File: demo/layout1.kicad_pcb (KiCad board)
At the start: 2 copper layers, 38 x 14 mm, 28 parts, among them J1 MICRO-USB-B-alt, P1 CONN_01X06, U1 FTDI-FT230X, U2 MCP1703-alt

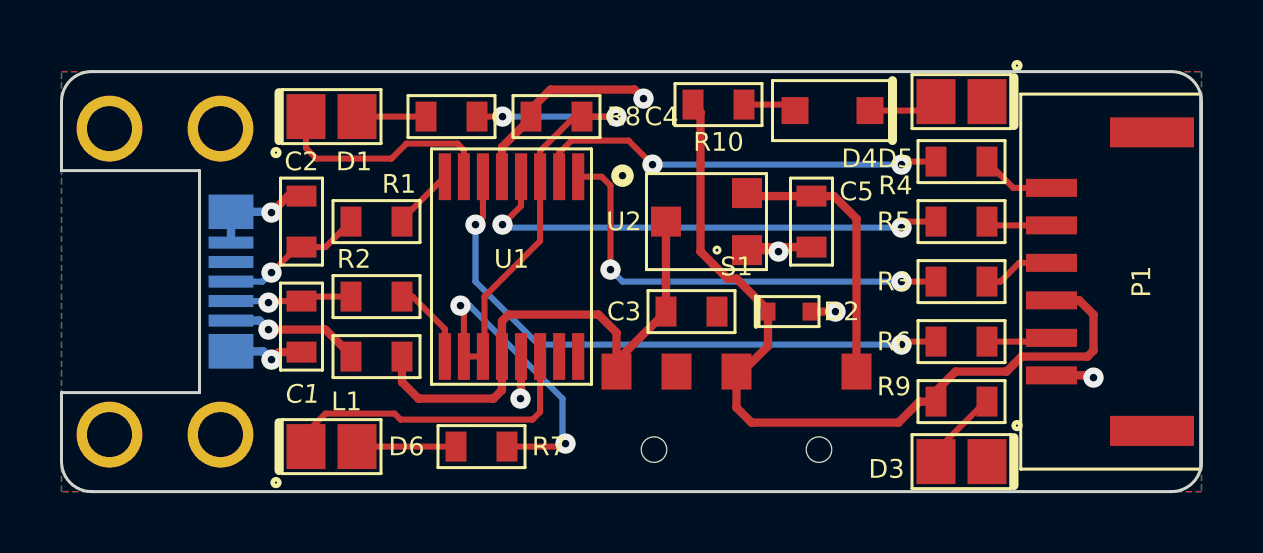
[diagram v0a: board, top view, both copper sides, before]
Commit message: lots of changes, can recenter placement,etc
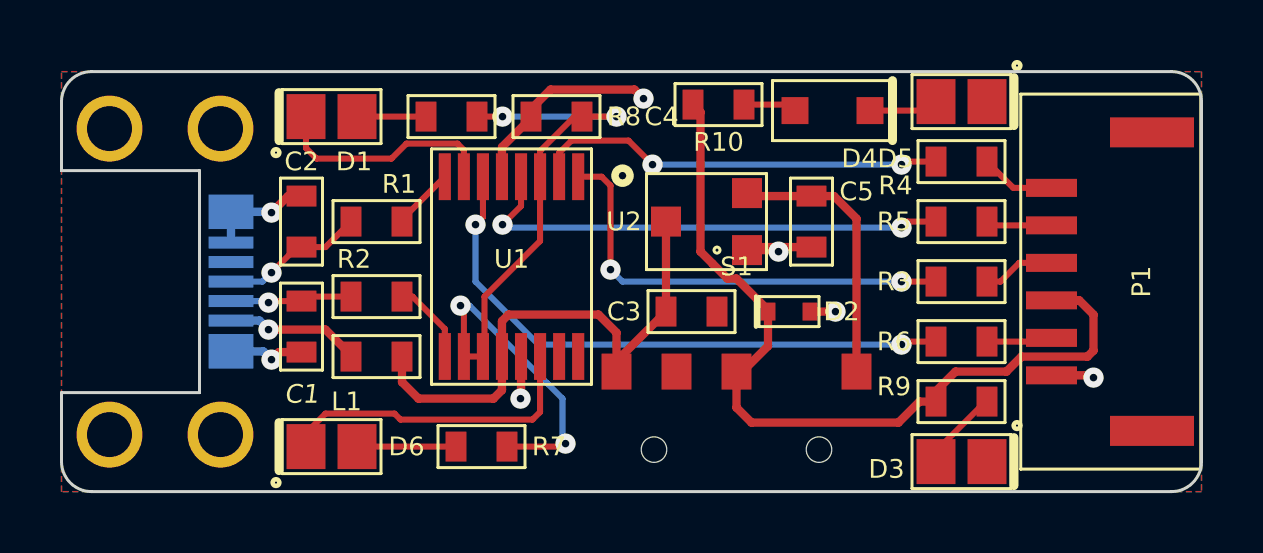
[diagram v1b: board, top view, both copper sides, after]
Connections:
- net /~CTS renamed /~{CTS}
- net /~CTS2 renamed /~{CTS2}
- net /~RTS renamed /~{RTS}
- net /~RTS2 renamed /~{RTS2}
- net /~RXLED renamed /~{RXLED}
- net /~RXLED2 renamed /~{RXLED2}
- net /~TXLED renamed /~{TXLED}
- net /~TXLED2 renamed /~{TXLED2}
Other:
- net class 50Ohm removed
- net class Default removed
- net class High-Power removed
- net class Power removed
- net class pull removed
